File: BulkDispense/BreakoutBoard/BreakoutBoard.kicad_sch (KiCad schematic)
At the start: 35 parts, among them J1 BS1, J10 OS3, J11 OS4, J12 FS1, J13 FS3, J14 PCV, J15 FS2, J16 FS4, J17 WL1, J18 WL2, J19 Analog Inputs, J2 BS2, J20 R0~R3, J21 R4~R7, J22 R8~R9, J23 Digital IN + R0~R4, J24 WB1, J25 WB2, J26 Digital Outputs, J27 R4~R9, J28 WV1, J29 WV2, J3 OS1, J30 Flow Sensors, J4 OS2, J5 PS, J6 MV1&2, J7 MV3&4, J8 BS3, J9 BS4

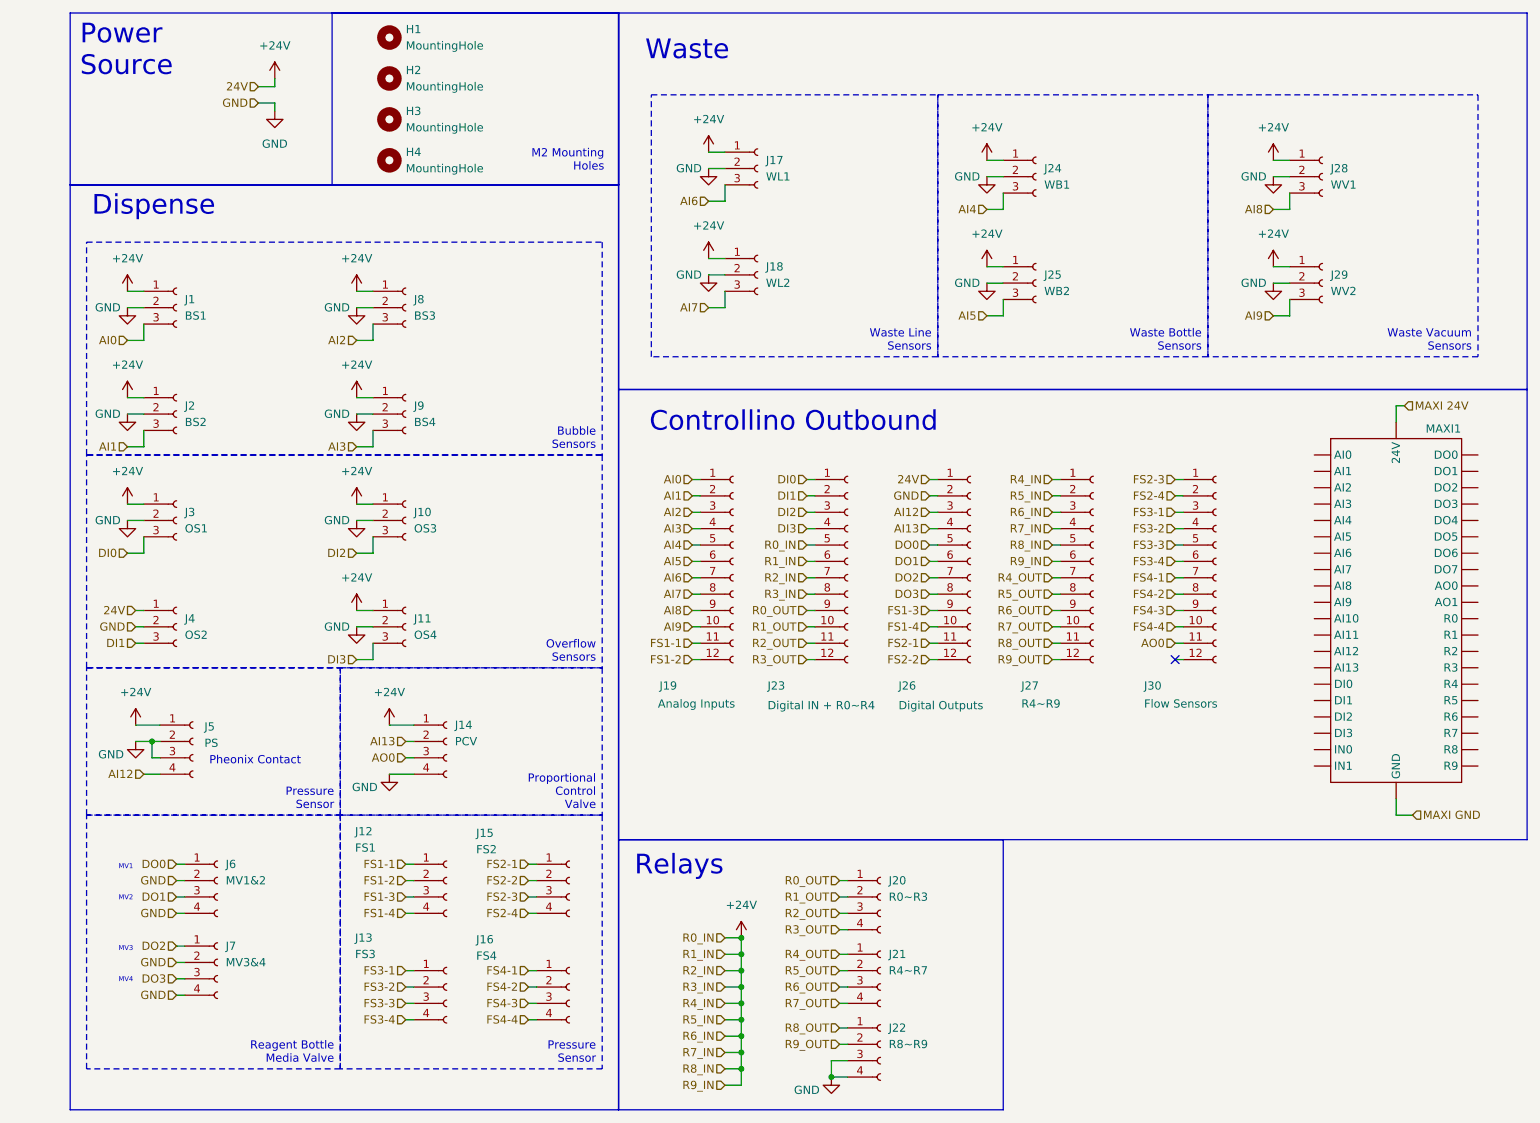
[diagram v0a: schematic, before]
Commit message: Design Overhaul
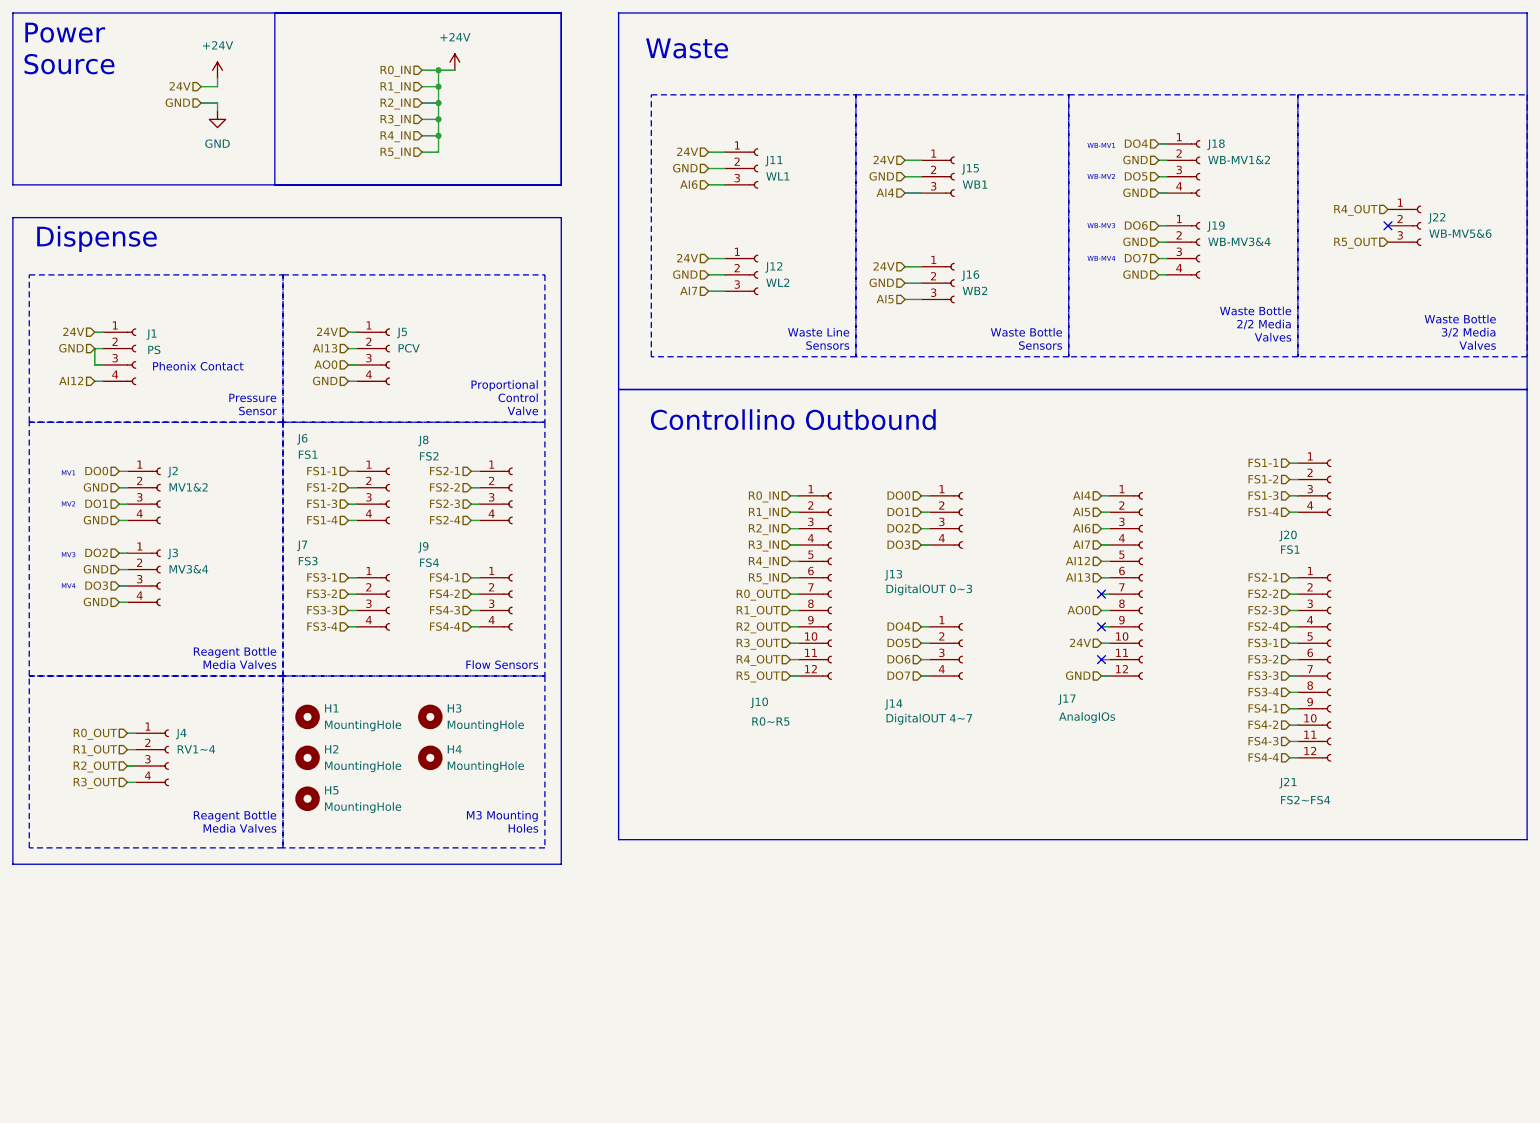
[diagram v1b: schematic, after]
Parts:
- removed J1: BS1, PartsLibrary:3720362A3003PL, symbol Connector:Conn_01x03_Socket
- removed J10: OS3, PartsLibrary:3720362A3003PL, symbol Connector:Conn_01x03_Socket
- removed J11: OS4, PartsLibrary:3720362A3003PL, symbol Connector:Conn_01x03_Socket
- removed J19: Analog Inputs, PartsLibrary:CONN_37212-62M3-003PL_3MM, symbol Connector:Conn_01x12_Socket
- removed J2: BS2, PartsLibrary:3720362A3003PL, symbol Connector:Conn_01x03_Socket
- removed J21: R4~R7, PartsLibrary:CONN_37204-62A3-004PL_3MM, symbol Connector:Conn_01x04_Socket
- removed J22: R8~R9, PartsLibrary:CONN_37204-62A3-004PL_3MM, symbol Connector:Conn_01x04_Socket
- removed J26: Digital Outputs, PartsLibrary:CONN_37212-62M3-003PL_3MM, symbol Connector:Conn_01x12_Socket
- removed J28: WV1, PartsLibrary:3720362A3003PL, symbol Connector:Conn_01x03_Socket
- removed J29: WV2, PartsLibrary:3720362A3003PL, symbol Connector:Conn_01x03_Socket
- removed J3: OS1, PartsLibrary:3720362A3003PL, symbol Connector:Conn_01x03_Socket
- removed J4: OS2, PartsLibrary:3720362A3003PL, symbol Connector:Conn_01x03_Socket
- removed J8: BS3, PartsLibrary:3720362A3003PL, symbol Connector:Conn_01x03_Socket
- removed J9: BS4, PartsLibrary:3720362A3003PL, symbol Connector:Conn_01x03_Socket
- removed MAXI1: ~, symbol SymbolLibrary:Controllino_MAXI
- added H5: MountingHole, MountingHole:MountingHole_3.2mm_M3, symbol Mechanical:MountingHole
- added J13: DigitalOUT 0~3, PartsLibrary:CONN_37204-62A3-004PL_3MM, symbol Connector:Conn_01x04_Socket
- added J14: DigitalOUT 4~7, PartsLibrary:CONN_37204-62A3-004PL_3MM, symbol Connector:Conn_01x04_Socket
- added J18: WB-MV1&2, PartsLibrary:CONN_37204-62A3-004PL_3MM, symbol Connector:Conn_01x04_Socket
- added J19: WB-MV3&4, PartsLibrary:CONN_37204-62A3-004PL_3MM, symbol Connector:Conn_01x04_Socket
- added J20: FS1, PartsLibrary:CONN_37204-62A3-004PL_3MM, symbol Connector:Conn_01x04_Socket
- added J22: WB-MV5&6, PartsLibrary:3720362A3003PL, symbol Connector:Conn_01x03_Socket
- H1, H2, H3, H4: footprint MountingHole:MountingHole_2.2mm_M2 -> MountingHole:MountingHole_3.2mm_M3
- J10: renamed from J23; value Digital IN + R0~R4 -> R0~R5
- J17: renamed from J27; value R4~R9 -> AnalogIOs
- J21: renamed from J30; value Flow Sensors -> FS2~FS4
- J4: renamed from J20; value R0~R3 -> RV1~4
- renumbered J5 to J1, J17 to J11, J18 to J12, J24 to J15, J25 to J16, J6 to J2, J7 to J3, J14 to J5, J12 to J6, J13 to J7, J15 to J8, J16 to J9
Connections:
- net DI0 is gone; now on net +24V: J10.1 (Pin_1)
- net DI1 is gone; now on net +24V: J10.2 (Pin_2)
- net DI2 is gone; now on net +24V: J10.3 (Pin_3)
- net DI3 is gone; now on net +24V: J10.4 (Pin_4)
- net R7_OUT is gone; now on net +24V: J17.10 (Pin_10)
- net R9_OUT is gone; now on net GND: J17.12 (Pin_12)
- net +24V: no longer J10.7 (Pin_7), J10.8 (Pin_8), J17.1 (Pin_1), J17.2 (Pin_2), J17.3 (Pin_3), J17.4 (Pin_4), J17.5 (Pin_5), J17.6 (Pin_6)
- net AI12: now also J17.5 (Pin_5)
- net AI13: now also J17.6 (Pin_6)
- net AI4: now also J17.1 (Pin_1)
- net AI5: now also J17.2 (Pin_2)
- net AI6: now also J17.3 (Pin_3)
- net AI7: now also J17.4 (Pin_4)
- net AO0: now also J17.8 (Pin_8); no longer J21.11 (Pin_11)
- net DO0: now also J13.1 (Pin_1)
- net DO1: now also J13.2 (Pin_2)
- net DO2: now also J13.3 (Pin_3)
- net DO3: now also J13.4 (Pin_4)
- net FS1-1: now also J20.1 (Pin_1)
- net FS1-2: now also J20.2 (Pin_2)
- net FS1-3: now also J20.3 (Pin_3)
- net FS1-4: now also J20.4 (Pin_4)
- net FS2-1: now also J21.1 (Pin_1)
- net FS2-2: now also J21.2 (Pin_2)
- net FS2-3: now also J21.3 (Pin_3); no longer J21.1 (Pin_1)
- net FS2-4: now also J21.4 (Pin_4); no longer J21.2 (Pin_2)
- net FS3-1: now also J21.5 (Pin_5); no longer J21.3 (Pin_3)
- net FS3-2: now also J21.6 (Pin_6); no longer J21.4 (Pin_4)
- net FS3-3: now also J21.7 (Pin_7); no longer J21.5 (Pin_5)
- net FS3-4: now also J21.8 (Pin_8); no longer J21.6 (Pin_6)
- net FS4-1: now also J21.9 (Pin_9); no longer J21.7 (Pin_7)
- net FS4-2: now also J21.10 (Pin_10); no longer J21.8 (Pin_8)
- net FS4-3: now also J21.11 (Pin_11); no longer J21.9 (Pin_9)
- net FS4-4: now also J21.12 (Pin_12); no longer J21.10 (Pin_10)
- net GND: now also J18.2 (Pin_2), J18.4 (Pin_4), J19.2 (Pin_2), J19.4 (Pin_4)
- net R0_OUT: now also J10.7 (Pin_7); no longer J10.9 (Pin_9)
- net R1_OUT: now also J10.8 (Pin_8); no longer J10.10 (Pin_10)
- net R2_OUT: now also J10.9 (Pin_9); no longer J10.11 (Pin_11)
- net R3_OUT: now also J10.10 (Pin_10); no longer J10.12 (Pin_12)
- net R4_OUT: now also J10.11 (Pin_11), J22.1 (Pin_1); no longer J17.7 (Pin_7)
- net R5_OUT: now also J10.12 (Pin_12), J22.3 (Pin_3); no longer J17.8 (Pin_8)
- net R6_OUT: no longer names the net of J17.9 (Pin_9)
- net R8_OUT: no longer names the net of J17.11 (Pin_11)
- new net DO4: J14.1 (Pin_1), J18.1 (Pin_1)
- new net DO5: J14.2 (Pin_2), J18.3 (Pin_3)
- new net DO6: J14.3 (Pin_3), J19.1 (Pin_1)
- new net DO7: J14.4 (Pin_4), J19.3 (Pin_3)
- no-connect marks 1 -> 4
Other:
- note added: "WB-MV1"
- note added: "WB-MV2"
- note added: "WB-MV3"
- note added: "WB-MV4"
- note removed: "Relays"
- moved on the sheet: J1, J10, J15, J16, J17, J2, J21, J3, J4, J5, J6, J7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
